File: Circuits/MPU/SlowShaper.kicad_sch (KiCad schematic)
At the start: 34 parts, among them U22 ADA4805-2ARMZ, U23 ADA4805-2ARMZ

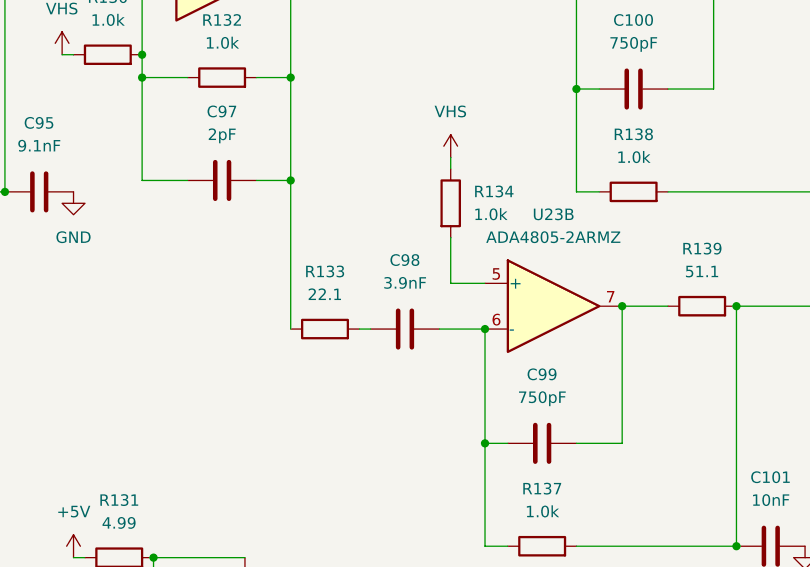
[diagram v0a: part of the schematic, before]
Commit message: revert cap changes from sim. Don't trust it...
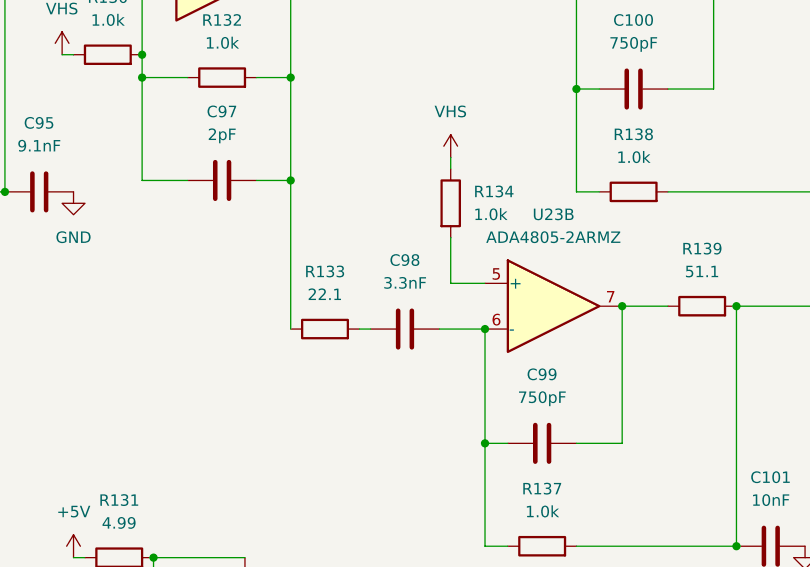
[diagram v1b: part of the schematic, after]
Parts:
- C98: value 3.9nF -> 3.3nF
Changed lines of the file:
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@@
 			)
 		)
-		(property "Value" "3.9nF"
+		(property "Value" "3.3nF"
 			(at 149.86 102.87 90)
 			(effects
